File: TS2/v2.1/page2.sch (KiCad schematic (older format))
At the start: 6 parts, among them U10 74LS32, U19 74LS20, U24 74LS260, U25 74LS260, U26 74LS138, U27 25LS2548

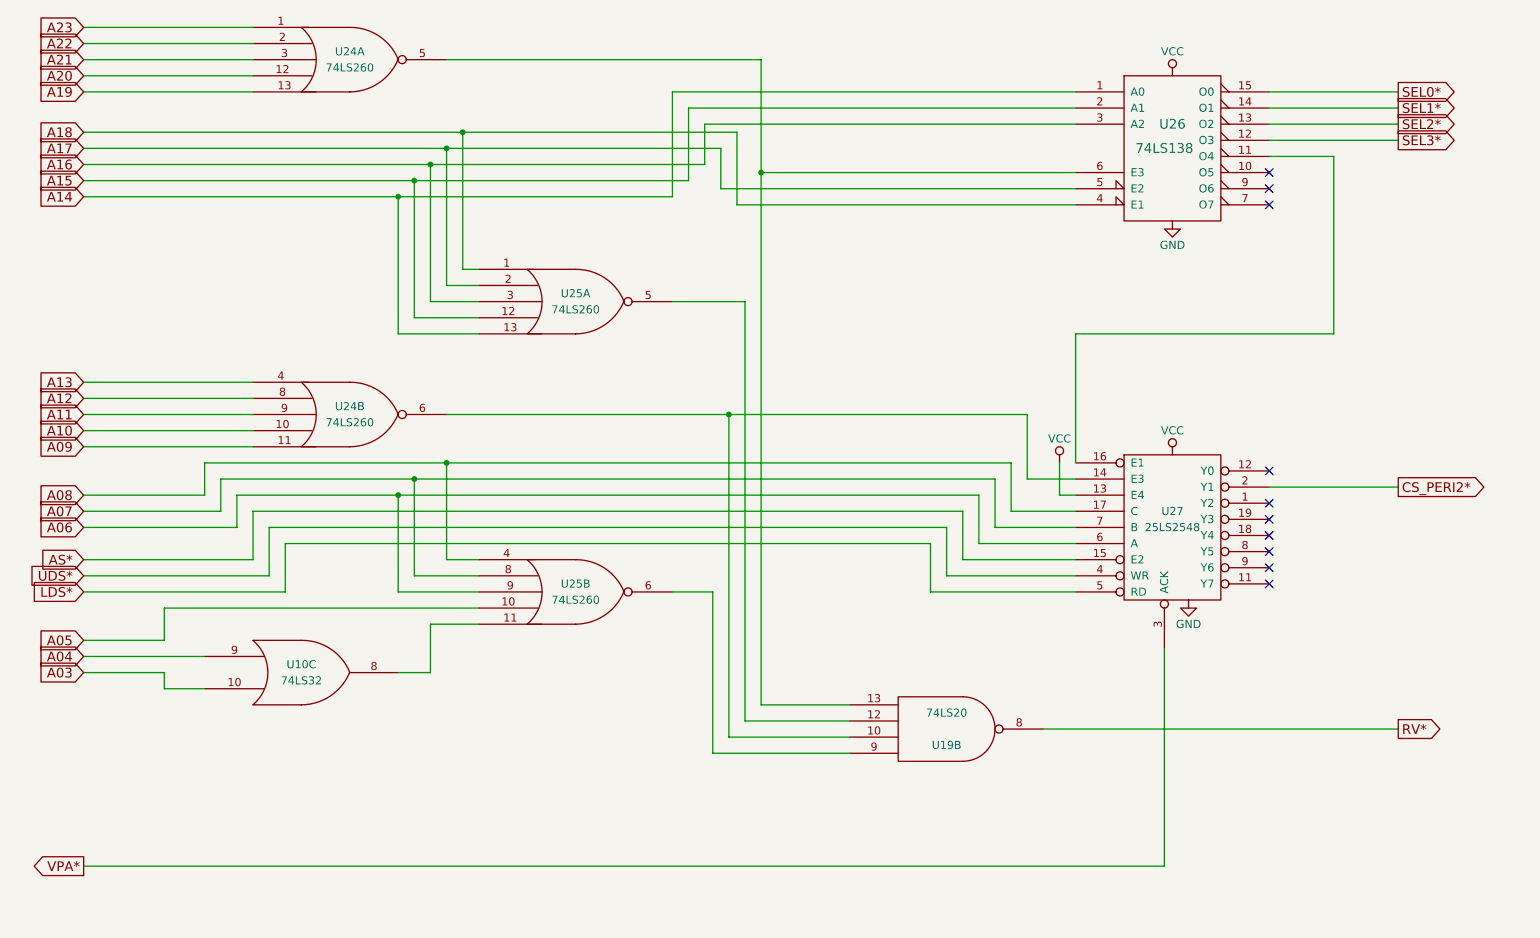
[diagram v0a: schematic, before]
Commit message: Rev 2.1 design changes.
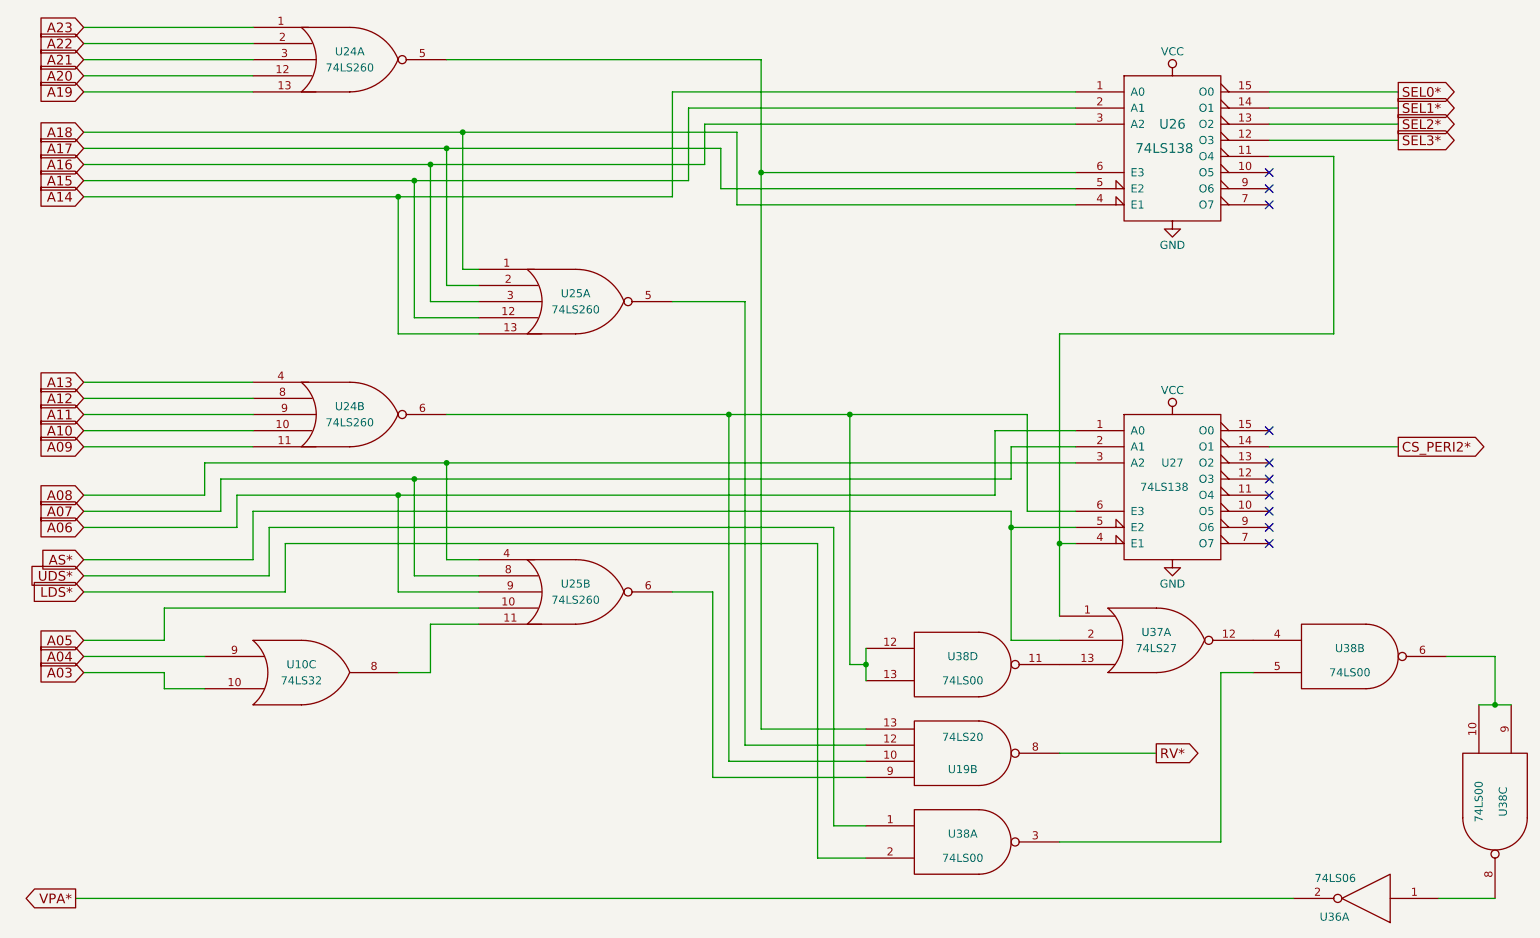
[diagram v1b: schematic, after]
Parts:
- removed U27: 25LS2548, Housings_DIP:DIP-20_W7.62mm, symbol 25LS2548
- added U27: 74LS138, Housings_DIP:DIP-16_W7.62mm, symbol 74LS138
- added U36: 74LS06, Housings_DIP:DIP-14_W7.62mm, symbol 74LS06
- added U37: 74LS27, Housings_DIP:DIP-14_W7.62mm, symbol 74LS27
- added U38: 74LS00, Housings_DIP:DIP-14_W7.62mm, symbol 74LS00
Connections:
- net A06: now also U27.1 (A0)
- net A07: now also U27.2 (A1)
- net A08: now also U27.3 (A2)
- net AS*: now also U27.5 (E2), U37.2
- net CS_PERI2*: now also U27.14 (O1)
- net GND: now also U27.8 (GND), U36.7 (GND), U37.7 (GND), U38.7 (GND), U38.7 (GND), U38.7 (GND), U38.7 (GND)
- net LDS*: now also U38.2
- net UDS*: now also U38.1
- net VCC: now also U27.16 (VCC), U36.14 (VCC), U37.14 (VCC), U38.14 (VCC), U38.14 (VCC), U38.14 (VCC), U38.14 (VCC)
- net VPA*: now also U36.2
- net at U26.11 (O4): now also U27.4 (E1), U37.1
- net at U19.10, U24.6: now also U27.6 (E3), U38.12, U38.13
- new net: U37.12, U38.4
- new net: U37.13, U38.11
- new net: U38.3, U38.5
- new net: U38.10, U38.6, U38.9
- new net: U36.1, U38.8
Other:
- moved on the sheet: U19B
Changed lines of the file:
@@
 Sheet 3 9
 Title "TS2 68000 Single Board Computer"
-Date "2017-02-12"
+Date "2017-02-14"
 Rev "2.1"
 Comp "Jeff Tranter"
@@
 L 74LS20 U19
 U 2 1 57BFBD6F
-P 6500 5350
-F 0 "U19" H 6500 5450 50  0000 C CNN
-F 1 "74LS20" H 6500 5250 50  0000 C CNN
-F 2 "Housings_DIP:DIP-14_W7.62mm" H 6500 5350 50  0001 C CNN
-F 3 "" H 6500 5350 50  0000 C CNN
-	2    6500 5350
+P 6600 5500
+F 0 "U19" H 6600 5600 50  0000 C CNN
+F 1 "74LS20" H 6600 5400 50  0000 C CNN
+F 2 "Housings_DIP:DIP-14_W7.62mm" H 6600 5500 50  0001 C CNN
+F 3 "" H 6600 5500 50  0000 C CNN
+	2    6600 5500
 	1    0    0    1
 $EndComp
@@
 F 3 "" H 4200 4500 50  0000 C CNN
 	2    4200 4500
-	1    0    0    -1
-$EndComp
-$Comp
-L 25LS2548 U27
-U 1 1 57C0FF1F
-P 7900 4100
-F 0 "U27" H 7900 4200 50  0000 C CNN
-F 1 "25LS2548" H 7900 4100 50  0000 C CNN
-F 2 "Housings_DIP:DIP-20_W7.62mm" H 7900 4100 50  0001 C CNN
-F 3 "" H 7900 4100 50  0000 C CNN
-	1    7900 4100
 	1    0    0    -1
 $EndComp
@@
 	3400 1200 5350 1200
 Wire Wire Line
-	5350 1200 5350 5200
+	5350 1200 5350 5350
 Wire Wire Line
 	5350 1900 7300 1900
@@
 Text GLabel 1150 5000 0    60   Input ~ 0
 A03
-Text GLabel 1150 6200 0    60   Output ~ 0
+Text GLabel 1100 6400 0    60   Output ~ 0
 VPA*
 Wire Wire Line
@@
 $EndComp
 Wire Wire Line
-	7300 3700 7300 2900
-Wire Wire Line
-	7300 2900 8900 2900
+	7200 2900 8900 2900
 Wire Wire Line
 	8900 2900 8900 1800
-Text GLabel 9300 3850 2    60   Output ~ 0
+Text GLabel 9300 3600 2    60   Output ~ 0
 CS_PERI2*
-NoConn ~ 8500 4050
-NoConn ~ 8500 4150
-NoConn ~ 8500 4250
-NoConn ~ 8500 4350
-NoConn ~ 8500 4450
+NoConn ~ 8500 3700
+NoConn ~ 8500 3800
+NoConn ~ 8500 3900
+NoConn ~ 8500 4000
+NoConn ~ 8500 4100
 $Comp
 L GND #PWR041
 U 1 1 57C1E717
-P 8000 4550
-F 0 "#PWR041" H 8000 4300 50  0001 C CNN
-F 1 "GND" H 8000 4400 50  0000 C CNN
-F 2 "" H 8000 4550 50  0000 C CNN
-F 3 "" H 8000 4550 50  0000 C CNN
-	1    8000 4550
+P 7900 4300
+F 0 "#PWR041" H 7900 4050 50  0001 C CNN
+F 1 "GND" H 7900 4150 50  0000 C CNN
+F 2 "" H 7900 4300 50  0000 C CNN
+F 3 "" H 7900 4300 50  0000 C CNN
+	1    7900 4300
 	1    0    0    -1
 $EndComp
@@
 L VCC #PWR042
 U 1 1 57C1E73D
-P 7900 3650
-F 0 "#PWR042" H 7900 3500 50  0001 C CNN
-F 1 "VCC" H 7900 3800 50  0000 C CNN
-F 2 "" H 7900 3650 50  0000 C CNN
-F 3 "" H 7900 3650 50  0000 C CNN
-	1    7900 3650
-	1    0    0    -1
-$EndComp
-Wire Wire Line
-	7850 6200 7850 4850
-Wire Wire Line
-	7100 5350 9300 5350
-Text GLabel 9300 5350 2    60   Output ~ 0
+P 7900 3400
+F 0 "#PWR042" H 7900 3250 50  0001 C CNN
+F 1 "VCC" H 7900 3550 50  0000 C CNN
+F 2 "" H 7900 3400 50  0000 C CNN
+F 3 "" H 7900 3400 50  0000 C CNN
+	1    7900 3400
+	1    0    0    -1
+$EndComp
+Text GLabel 7800 5500 2    60   Output ~ 0
 RV*
 Wire Wire Line
-	7300 4300 6600 4300
-Wire Wire Line
-	6600 4300 6600 4000
-Wire Wire Line
-	6600 4000 2200 4000
+	6900 4000 2200 4000
 Wire Wire Line
 	2200 4000 2200 4300
@@
 	2300 4400 2300 4100
 Wire Wire Line
-	2300 4100 6500 4100
-Wire Wire Line
-	6500 4100 6500 4400
-Wire Wire Line
-	6500 4400 7300 4400
-Wire Wire Line
-	7300 4500 6400 4500
-Wire Wire Line
-	6400 4500 6400 4200
-Wire Wire Line
-	6400 4200 2400 4200
-Wire Wire Line
 	2400 4200 2400 4500
 Wire Wire Line
@@
 	2100 4100 2100 3900
 Wire Wire Line
-	2100 3900 6700 3900
-Wire Wire Line
-	6700 3900 6700 4200
-Wire Wire Line
-	6700 4200 7300 4200
+	2100 3900 6800 3900
 Wire Wire Line
 	1150 4000 2000 4000
@@
 	2000 4000 2000 3800
 Wire Wire Line
-	2000 3800 6800 3800
-Wire Wire Line
-	6800 3800 6800 4100
-Wire Wire Line
-	6800 4100 7300 4100
+	2000 3800 6900 3800
 Wire Wire Line
 	1150 3900 1900 3900
@@
 	1900 3900 1900 3700
 Wire Wire Line
-	1900 3700 6900 3700
-Wire Wire Line
-	6900 3700 6900 4000
-Wire Wire Line
-	6900 4000 7300 4000
-Wire Wire Line
-	7300 3800 7000 3800
-Wire Wire Line
-	7000 3800 7000 3400
-Wire Wire Line
-	7000 3400 3400 3400
-Wire Wire Line
-	7300 3900 7200 3900
-Wire Wire Line
-	7200 3900 7200 3700
-$Comp
-L VCC #PWR043
-U 1 1 57C1EB1C
-P 7200 3700
-F 0 "#PWR043" H 7200 3550 50  0001 C CNN
-F 1 "VCC" H 7200 3850 50  0000 C CNN
-F 2 "" H 7200 3700 50  0000 C CNN
-F 3 "" H 7200 3700 50  0000 C CNN
-	1    7200 3700
-	1    0    0    -1
-$EndComp
+	1900 3700 7300 3700
+Wire Wire Line
+	3400 3400 7000 3400
 Wire Wire Line
 	1150 1650 5200 1650
@@
 	4800 4500 5050 4500
 Wire Wire Line
-	5050 4500 5050 5500
-Wire Wire Line
-	5050 5500 5900 5500
-Wire Wire Line
-	5900 5400 5150 5400
-Wire Wire Line
-	5150 5400 5150 3400
+	5050 4500 5050 5650
+Wire Wire Line
+	5050 5650 6000 5650
+Wire Wire Line
+	5150 5550 6000 5550
+Wire Wire Line
+	5150 3400 5150 5550
 Connection ~ 5150 3400
 Wire Wire Line
-	5900 5300 5250 5300
-Wire Wire Line
-	5250 5300 5250 2700
+	5250 5450 6000 5450
+Wire Wire Line
+	5250 2700 5250 5450
 Wire Wire Line
 	5250 2700 4800 2700
 Wire Wire Line
-	5350 5200 5900 5200
+	5350 5350 6000 5350
 Connection ~ 5350 1900
 Wire Wire Line
@@
 Wire Wire Line
 	8900 1800 8500 1800
-NoConn ~ 8500 3950
-Wire Wire Line
-	7850 6200 1150 6200
-NoConn ~ 8500 3750
-Wire Wire Line
-	8500 3850 9300 3850
+NoConn ~ 8500 3500
+NoConn ~ 8500 4200
+$Comp
+L 74LS138 U27
+U 1 1 58A0C2DC
+P 7900 3850
+F 0 "U27" H 7900 4000 50  0000 C CNN
+F 1 "74LS138" H 7850 3850 50  0000 C CNN
+F 2 "Housings_DIP:DIP-16_W7.62mm" H 7900 3850 50  0001 C CNN
+F 3 "" H 7900 3850 50  0000 C CNN
+	1    7900 3850
+	1    0    0    -1
+$EndComp
+Wire Wire Line
+	7300 4200 7200 4200
+Wire Wire Line
+	7200 2900 7200 4650
+Wire Wire Line
+	6900 4000 6900 4800
+Wire Wire Line
+	6900 4100 7300 4100
+Wire Wire Line
+	7000 3400 7000 4000
+Wire Wire Line
+	7000 4000 7300 4000
+Wire Wire Line
+	8500 3600 9300 3600
+Wire Wire Line
+	6900 3800 6900 3600
+Wire Wire Line
+	6900 3600 7300 3600
+Wire Wire Line
+	6800 3900 6800 3500
+Wire Wire Line
+	6800 3500 7300 3500
+Connection ~ 7200 4200
+Wire Wire Line
+	6900 4800 7200 4800
+Connection ~ 6900 4100
+$Comp
+L 74LS27 U37
+U 1 1 58A2A873
+P 7800 4800
+F 0 "U37" H 7800 4850 50  0000 C CNN
+F 1 "74LS27" H 7800 4750 50  0000 C CNN
+F 2 "Housings_DIP:DIP-14_W7.62mm" H 7800 4800 50  0001 C CNN
+F 3 "" H 7800 4800 50  0000 C CNN
+	1    7800 4800
+	1    0    0    -1
+$EndComp
+$Comp
+L 74LS00 U38
+U 1 1 58A2B1D0
+P 6600 6050
+F 0 "U38" H 6600 6100 50  0000 C CNN
+F 1 "74LS00" H 6600 5950 50  0000 C CNN
+F 2 "Housings_DIP:DIP-14_W7.62mm" H 6600 6050 50  0001 C CNN
+F 3 "" H 6600 6050 50  0000 C CNN
+	1    6600 6050
+	1    0    0    -1
+$EndComp
+Wire Wire Line
+	5700 4200 5700 6150
+Wire Wire Line
+	5700 4200 2400 4200
+$Comp
+L 74LS00 U38
+U 2 1 58A2BB8F
+P 9000 4900
+F 0 "U38" H 9000 4950 50  0000 C CNN
+F 1 "74LS00" H 9000 4800 50  0000 C CNN
+F 2 "Housings_DIP:DIP-14_W7.62mm" H 9000 4900 50  0001 C CNN
+F 3 "" H 9000 4900 50  0000 C CNN
+	2    9000 4900
+	1    0    0    -1
+$EndComp
+Wire Wire Line
+	8400 5000 8200 5000
+Wire Wire Line
+	8200 5000 8200 6050
+Wire Wire Line
+	9600 4900 9900 4900
+Wire Wire Line
+	9900 4900 9900 5200
+$Comp
+L 74LS06 U36
+U 1 1 58A2C282
+P 9100 6400
+F 0 "U36" H 9295 6515 50  0000 C CNN
+F 1 "74LS06" H 9290 6275 50  0000 C CNN
+F 2 "Housings_DIP:DIP-14_W7.62mm" H 9100 6400 50  0001 C CNN
+F 3 "" H 9100 6400 50  0000 C CNN
+	1    9100 6400
+	-1   0    0    1
+$EndComp
+Wire Wire Line
+	9550 6400 9900 6400
+Wire Wire Line
+	8650 6400 1100 6400
+$Comp
+L 74LS00 U38
+U 3 1 58A3852D
+P 9900 5800
+F 0 "U38" H 9900 5850 50  0000 C CNN
+F 1 "74LS00" H 9900 5700 50  0000 C CNN
+F 2 "Housings_DIP:DIP-14_W7.62mm" H 9900 5800 50  0001 C CNN
+F 3 "" H 9900 5800 50  0000 C CNN
+	3    9900 5800
+	0    1    1    0
+$EndComp
+Wire Wire Line
+	9800 5200 10000 5200
+Connection ~ 9900 5200
+$Comp
+L 74LS00 U38
+U 4 1 58A38C2E
+P 6600 4950
+F 0 "U38" H 6600 5000 50  0000 C CNN
+F 1 "74LS00" H 6600 4850 50  0000 C CNN
+F 2 "Housings_DIP:DIP-14_W7.62mm" H 6600 4950 50  0001 C CNN
+F 3 "" H 6600 4950 50  0000 C CNN
+	4    6600 4950
+	1    0    0    -1
+$EndComp
+Wire Wire Line
+	6000 4850 6000 5050
+Wire Wire Line
+	5800 4100 5800 5950
+Wire Wire Line
+	2300 4100 5800 4100
+Wire Wire Line
+	6000 4950 5900 4950
+Wire Wire Line
+	5900 4950 5900 3400
+Connection ~ 5900 3400
+Connection ~ 6000 4950
+Wire Wire Line
+	5800 5950 6000 5950
+Wire Wire Line
+	5700 6150 6000 6150
+Wire Wire Line
+	8200 6050 7200 6050
+Wire Wire Line
+	7200 5500 7800 5500
 $EndSCHEMATC
